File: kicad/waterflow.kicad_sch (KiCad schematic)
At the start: 14 parts, among them J1 Terminal, Q1 BC547, Q2 BC547, Q3 AO4447, U1 WeMos_D1_mini

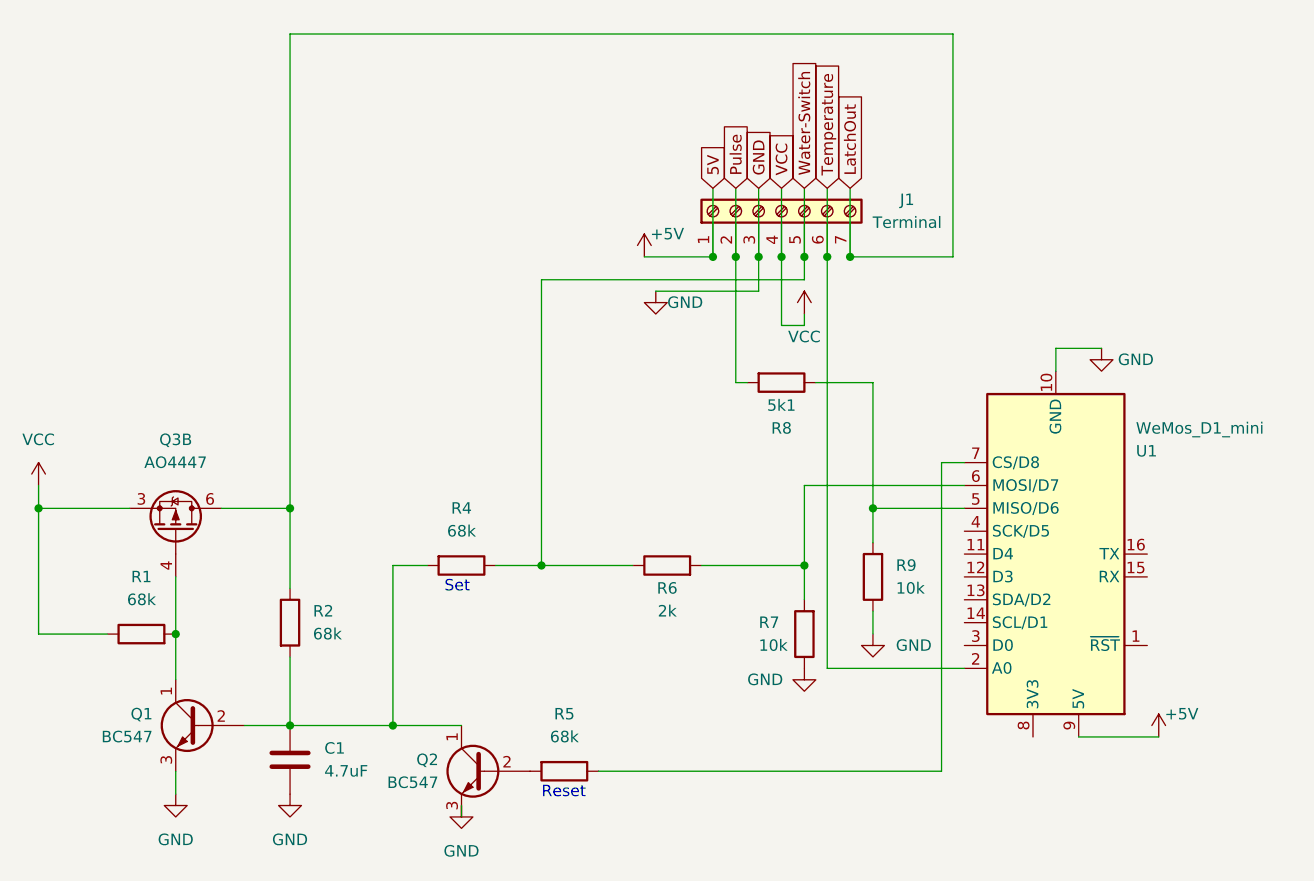
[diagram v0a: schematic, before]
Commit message: release v1.1
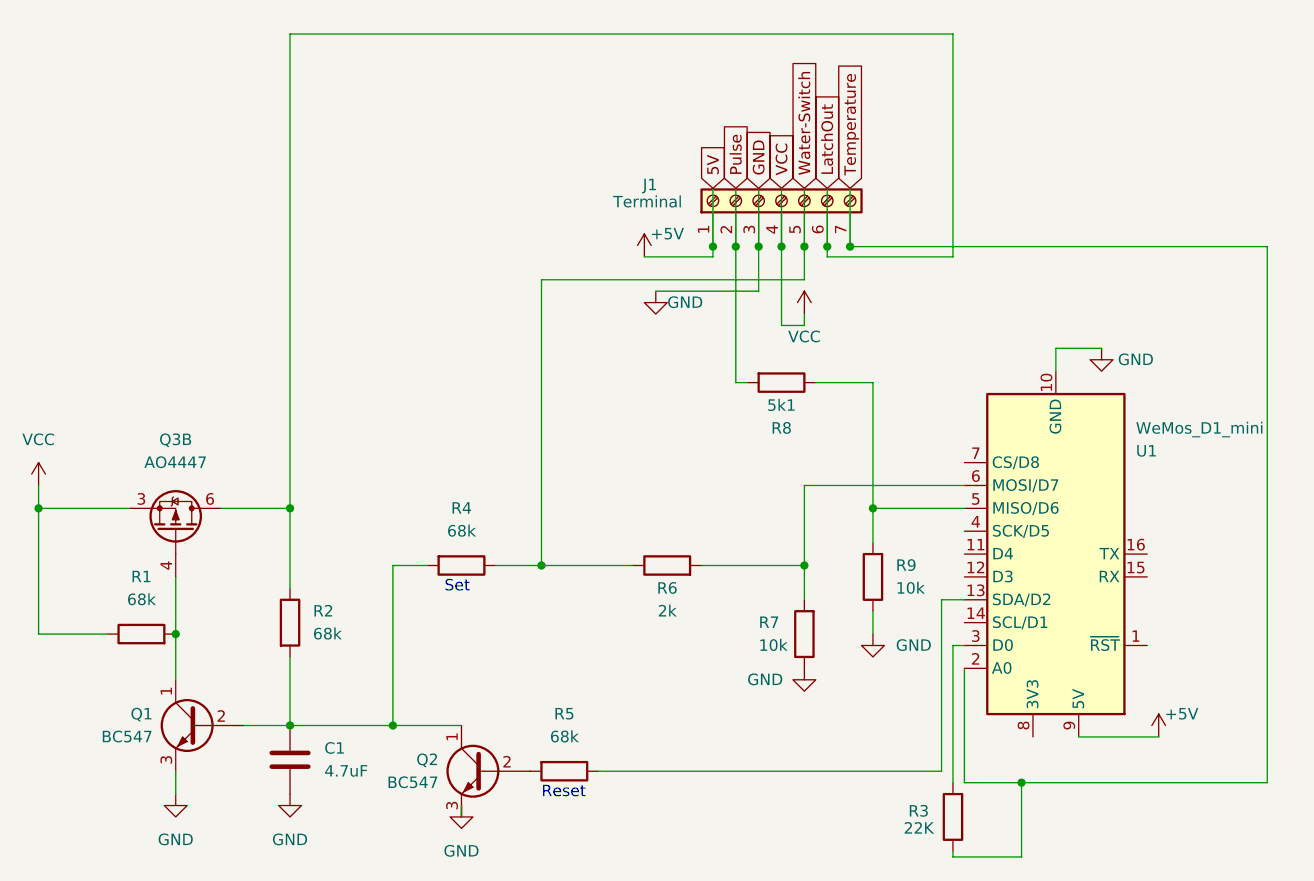
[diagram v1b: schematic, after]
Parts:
- added R3: 22K, Resistor_THT:R_Axial_DIN0207_L6.3mm_D2.5mm_P10.16mm_Horizontal, symbol Device:R
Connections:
- net LatchOut: now also J1.6 (Pin_6); no longer J1.7 (Pin_7)
- net Temperature: now also J1.7 (Pin_7), R3.1; no longer J1.6 (Pin_6)
- net at U1.13 (SDA/D2): now also R5.1
- net at U1.3 (D0): now also R3.2
- net at U1.7 (CS/D8): no longer R5.1
